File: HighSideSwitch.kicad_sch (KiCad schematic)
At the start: 24 parts, among them J1 Conn_02x02_Odd_Even, Q1 CSD18540Q5B, Q2 CSD18540Q5B, Q3 8050, U1 LM5060, U2 LM5050-1

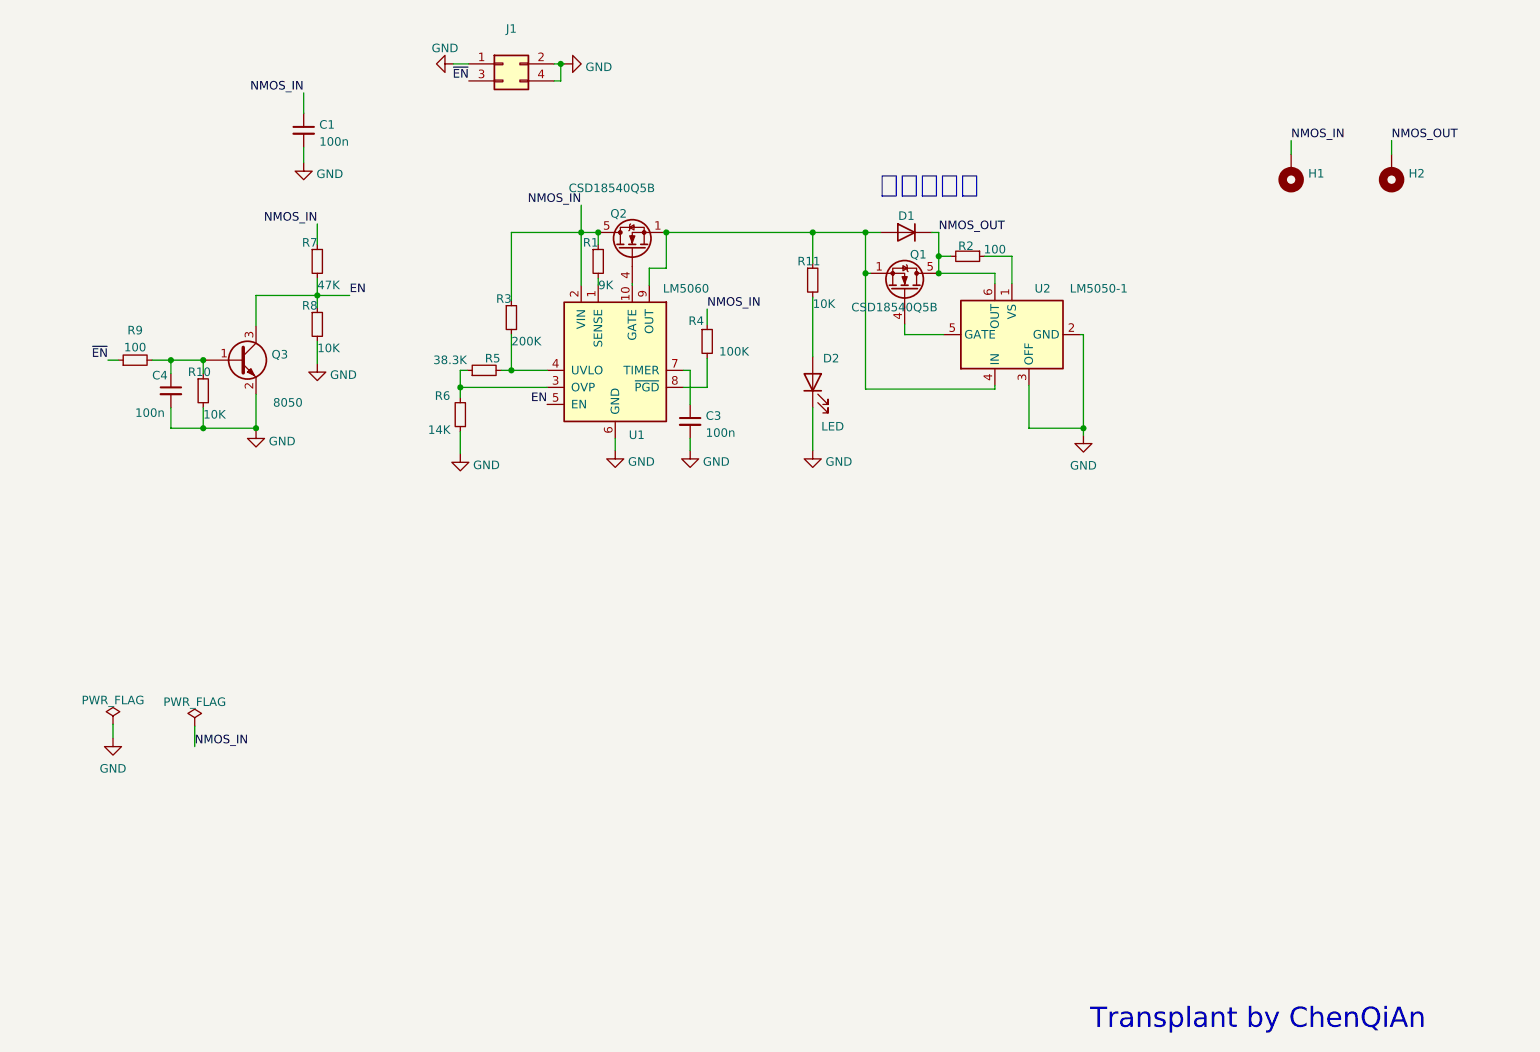
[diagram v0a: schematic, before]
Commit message: S
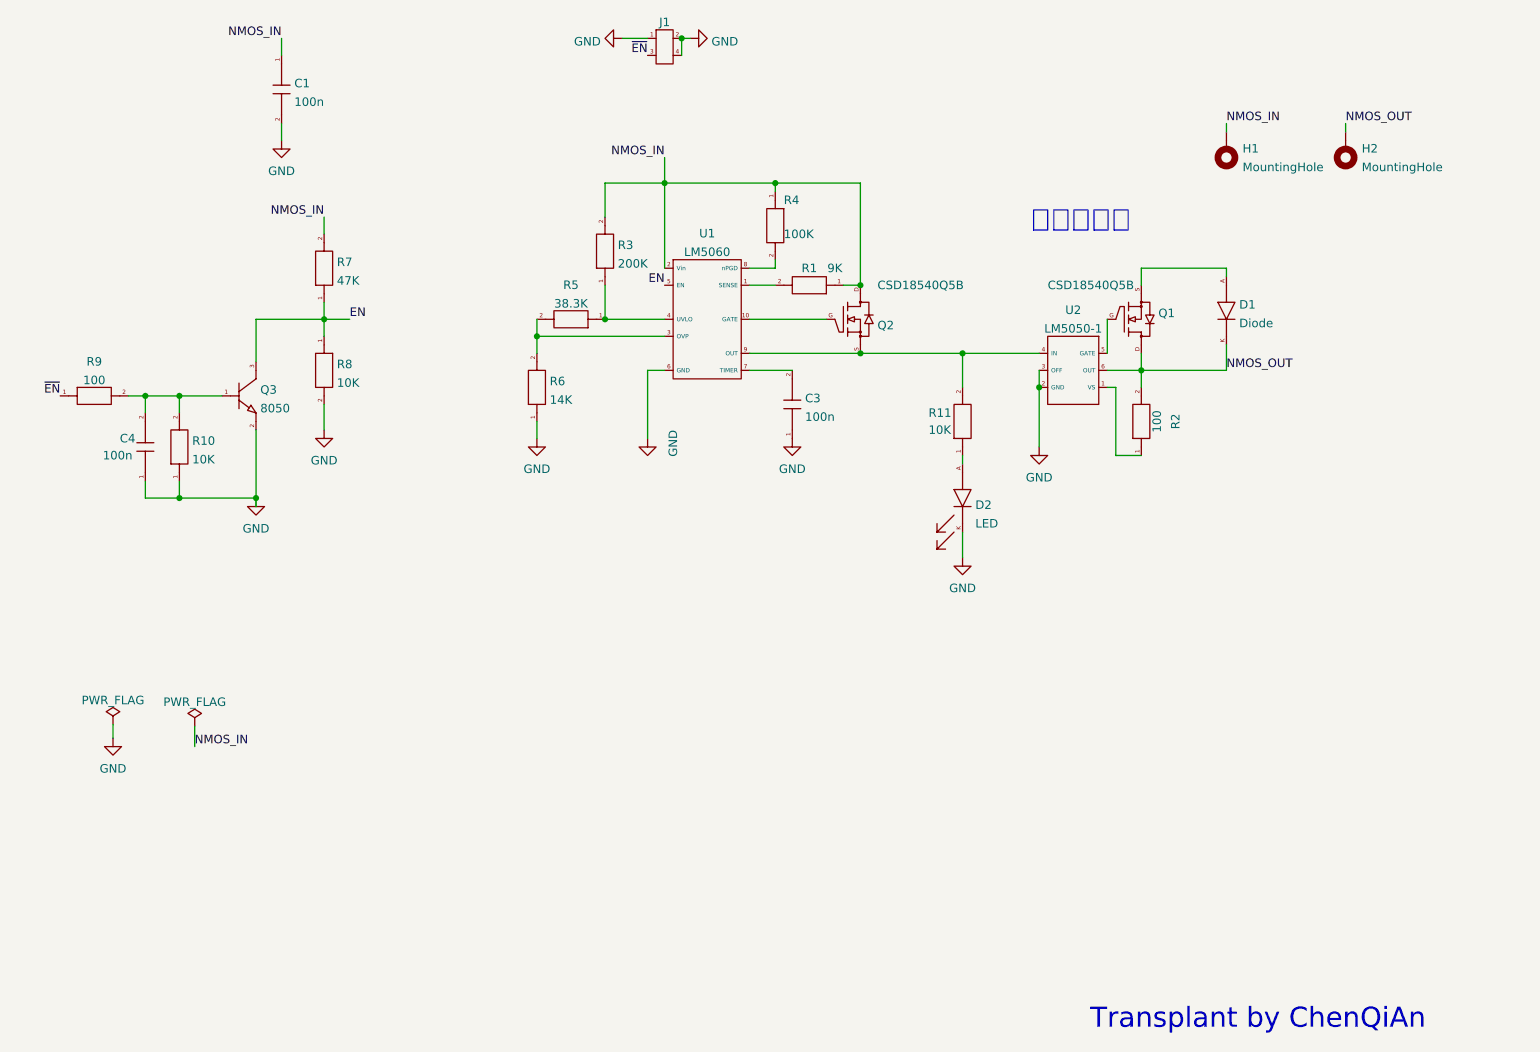
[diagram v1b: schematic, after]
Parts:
- removed C1, C3, C4: 100n, Capacitor_SMD:C_0402_1005Metric, symbol Device:C_Small
- removed D1: VS-6ESU06, Package_TO_SOT_SMD:TO-277A, symbol Diode:VS-6ESU06
- removed D2: LED, LED_SMD:LED_0603_1608Metric, symbol Device:LED
- removed H1, H2: MountingHole_Pad, MountingHole:MountingHole_3.2mm_M3_Pad_Via, symbol Mechanical:MountingHole_Pad
- removed J1: Conn_02x02_Odd_Even, Connector_PinHeader_1.27mm:PinHeader_2x02_P1.27mm_Vertical_SMD, symbol Connector_Generic:Conn_02x02_Odd_Even
- removed Q1, Q2: CSD18540Q5B, Package_TO_SOT_SMD:TDSON-8-1, symbol Transistor_FET:CSD18540Q5B
- removed Q3: 8050, Package_TO_SOT_SMD:TSOT-23, symbol Device:Q_NPN_BEC
- removed R1: 9K, Resistor_SMD:R_0402_1005Metric, symbol Device:R_Small
- removed R10, R11, R8: 10K, Resistor_SMD:R_0402_1005Metric, symbol Device:R_Small
- removed R2, R9: 100, Resistor_SMD:R_0402_1005Metric, symbol Device:R_Small
- removed R3: 200K, Resistor_SMD:R_0402_1005Metric, symbol Device:R_Small
- removed R4: 100K, Resistor_SMD:R_0402_1005Metric, symbol Device:R_Small
- removed R5: 38.3K, Resistor_SMD:R_0402_1005Metric, symbol Device:R_Small
- removed R6: 14K, Resistor_SMD:R_0402_1005Metric, symbol Device:R_Small
- removed R7: 47K, Resistor_SMD:R_0402_1005Metric, symbol Device:R_Small
- removed U1: LM5060, Package_SO:MSOP-10_3x3mm_P0.5mm, symbol Power_Management:LM5060
- removed U2: LM5050-1, Package_TO_SOT_SMD:TSOT-23-6, symbol Power_Management:LM5050-1
- added C1, C3, C4: 100n, GENERAL_RCL_SMD:C0402(1005M), symbol Basic_passive_components:Capacitor
- added D1: Diode, POWER_DIODE_SMD:TO-277A, symbol Power_diode:Diode
- added D2: LED, GENERAL_2-PIN_PLASTIC_SMD:LED0603(1608M), symbol Basic_passive_components:LED
- added H1, H2: MountingHole, MOUNTINGHOLE:MountingHole, symbol MountingHole:MountingHole
- added J1: Conn_02x02, CONNECTOR:Conn-02x02, symbol Link_W2B_connector:Conn_02x02
- added Q1, Q2: CSD18540Q5B, POWER_TRANSISTOR_SMD:SON-8_5x6_M, symbol Power_transistor:CSD18540Q5B
- added Q3: 8050, GENERAL_SMALL-SEMI_SMD:SOT-23, symbol Basic_semiconductor:BJT_NPN
- added R1: 9K, GENERAL_RCL_SMD:R0402(1005M), symbol Basic_passive_components:Resistor
- added R10, R11, R8: 10K, GENERAL_RCL_SMD:R0402(1005M), symbol Basic_passive_components:Resistor
- added R2, R9: 100, GENERAL_RCL_SMD:R0402(1005M), symbol Basic_passive_components:Resistor
- added R3: 200K, GENERAL_RCL_SMD:R0402(1005M), symbol Basic_passive_components:Resistor
- added R4: 100K, GENERAL_RCL_SMD:R0402(1005M), symbol Basic_passive_components:Resistor
- added R5: 38.3K, GENERAL_RCL_SMD:R0402(1005M), symbol Basic_passive_components:Resistor
- added R6: 14K, GENERAL_RCL_SMD:R0402(1005M), symbol Basic_passive_components:Resistor
- added R7: 47K, GENERAL_RCL_SMD:R0402(1005M), symbol Basic_passive_components:Resistor
- added U1: LM5060, GENERAL_MIDDLE-SEMI_SMD:MSOP-3030_10, symbol Integrated-circuit_transistor_driver:LM5060
- added U2: LM5050-1, GENERAL_SMALL-SEMI_SMD:SOT-23-6, symbol Integrated-circuit_transistor_driver:LM5050-1
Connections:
- net EN: now also Q3.3 (Collector), R7.1, R8.1, U1.5 (EN)
- net GND: now also C1.2, C3.1, C4.1, D2.K, J1.1, J1.2, J1.4, Q3.2 (Emitter), R10.1, R6.1, R8.2, U1.6 (GND), U2.2 (GND), U2.3 (OFF)
- net NMOS_IN: now also C1.1, H1., Q2.D (Drain), R1.1, R3.2, R4.1, R7.2, U1.2 (Vin)
- net NMOS_OUT: now also D1.K (Cathode), H2., Q1.D (Drain), R2.2, U2.6 (OUT)
- net ~{EN}: now also J1.3, R9.1
- new net: D1.A (Anode), Q1.S (Source)
- new net: R2.1, U2.1 (VS)
- new net: Q2.S (Source), R11.2, U1.9 (OUT), U2.4 (IN)
- new net: Q1.G (Gate), U2.5 (GATE)
- new net: R4.2, U1.8 (nPGD)
- new net: C4.2, Q3.1 (Base), R10.2, R9.2
- new net: R1.2, U1.1 (SENSE)
- new net: Q2.G (Gate), U1.10 (GATE)
- new net: R5.2, R6.2, U1.3 (OVP)
- new net: R3.1, R5.1, U1.4 (UVLO)
- new net: C3.2, U1.7 (TIMER)
- new net: D2.A, R11.1
